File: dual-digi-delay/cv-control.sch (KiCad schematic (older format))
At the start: 44 parts, among them Q3 2N3904, Q4 2N3904, Q5 2N3904, Q6 2N3904, U5 TL074, U6 TL074

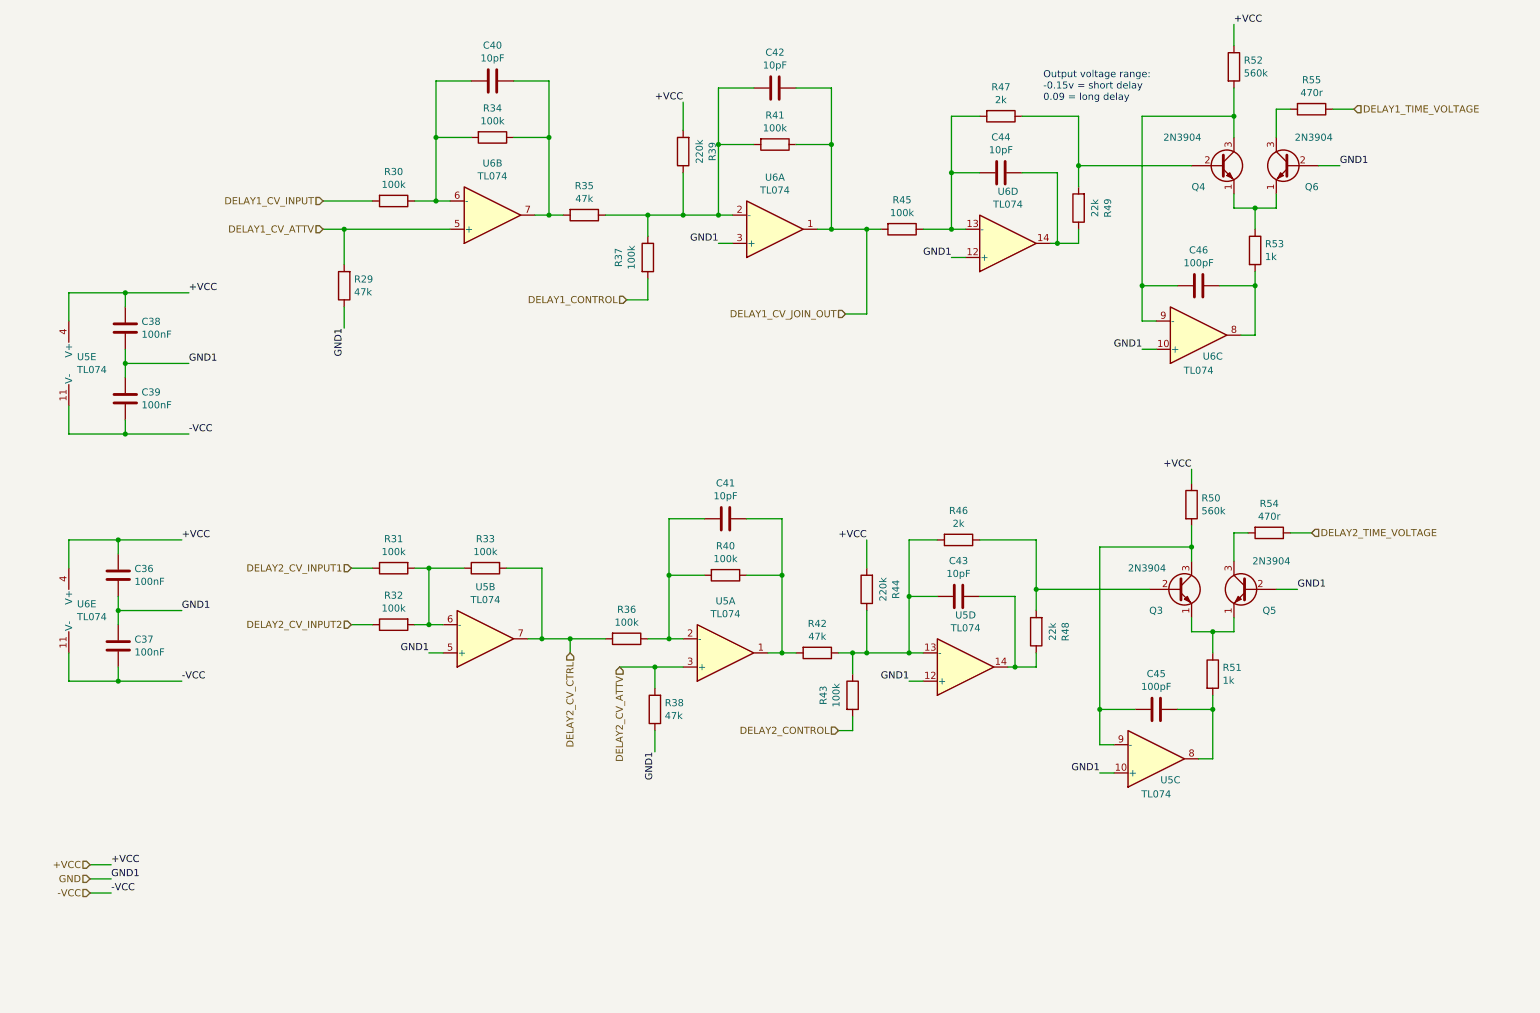
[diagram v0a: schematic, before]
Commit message: Final revision of dual digi delay
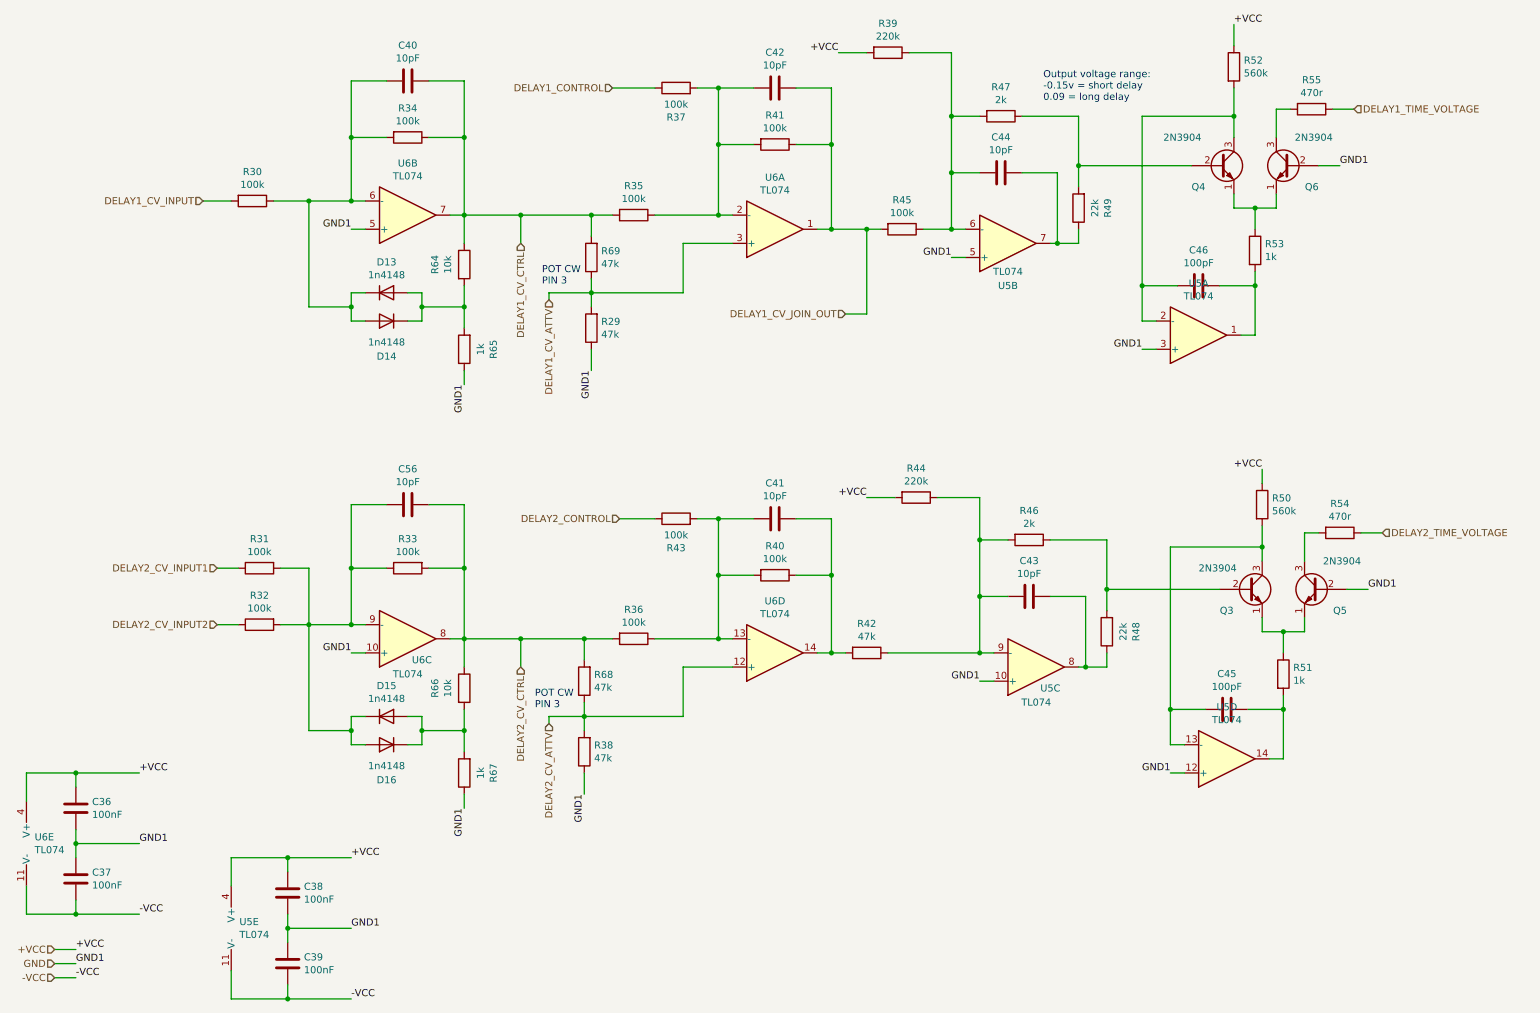
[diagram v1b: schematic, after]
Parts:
- added C56: 10pF, rumblesan-footprints:C_Rect_L7.0mm_W3.5mm_P5.00mm, symbol Device:C
- added D13, D14, D15, D16: 1n4148, rumblesan-footprints:Diode_THT_P7.62mm_Horizontal, symbol Device:D
- added R64, R66: 10k, rumblesan-footprints:Resistor_THT_L6.3mm_D2.5mm_P10.16mm_Horizontal, symbol Device:R
- added R65, R67: 1k, rumblesan-footprints:Resistor_THT_L6.3mm_D2.5mm_P10.16mm_Horizontal, symbol Device:R
- added R68, R69: 47k, rumblesan-footprints:Resistor_THT_L6.3mm_D2.5mm_P10.16mm_Horizontal, symbol Device:R
- R35: value 47k -> 100k
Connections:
- net DELAY1_CONTROL: now also R37.1; no longer R37.2
- net DELAY1_CV_ATTV: now also U6.3 (+), R69.1; no longer U6.5 (+)
- net DELAY2_CONTROL: now also R43.1; no longer R43.2
- net DELAY2_CV_ATTV: now also U6.12 (+), R68.1; no longer U5.3 (+)
- net DELAY2_CV_CTRL: now also U6.8, C56.1, R66.1, R68.2; no longer U5.7
- net GND: now also U5.3 (+), U6.5 (+), R65.1, R67.1; no longer U6.12 (+), U6.3 (+)
- net at R31.2, R32.2, R33.1: now also U6.9 (-), C56.2, D15.1 (K), D16.2 (A); no longer U5.6 (-)
- net at C45.2, R51.2: now also U5.14; no longer U5.8
- net at C45.1, Q3.3 (C), R50.2: now also U5.13 (-); no longer U5.9 (-)
- net at C43.2, R42.1, R44.1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: now also U5.9 (-); no longer R43.1, U5.13 (-)
- net at C43.1, R48.1: now also U5.8; no longer U5.14
- net at C41.1, R40.1, R42.2: now also U6.14; no longer U5.1
- net at C41.2, R36.1, R40.2: now also R43.2, U6.13 (-); no longer U5.2 (-)
- net at C40.2, R30.1, R34.2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: now also D13.1 (K), D14.2 (A)
- net DELAY1_CV_CTRL: now reaches C40.1, R34.1, R35.2, U6.7
- net DELAY1_CV_CTRL: now also R64.1, R69.2
- net at C46.2, R53.2: now also U5.1; no longer U6.8
- net at C46.1, Q4.3 (C), R52.2: now also U5.2 (-); no longer U6.9 (-)
- net at C44.2, R45.1, R47.2: now also R39.1, U5.6 (-); no longer U6.13 (-)
- net at C44.1, R49.1: now also U5.7; no longer U6.14
- net at C42.2, R35.1, R41.2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: now also R37.2; no longer R37.1, R39.1
- new net: D13.2 (A), D14.1 (K), R64.2, R65.2
- new net: D15.2 (A), D16.1 (K), R66.2, R67.2
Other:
- note added: "POT CW\nPIN 3"
- moved on the sheet: C36, C37, C38, C39, C40, C41, C43, C45, Q3, Q5, R29, R30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
